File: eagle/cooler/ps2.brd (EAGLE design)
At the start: 160 x 100 mm, 8 parts, among them J1 PIN2F061.100, J2 PIN2F061.100, J3 PIN2F061.100, J4 PIN2F061.100, J5 PIN2F061.100, J6 PIN2F061.100

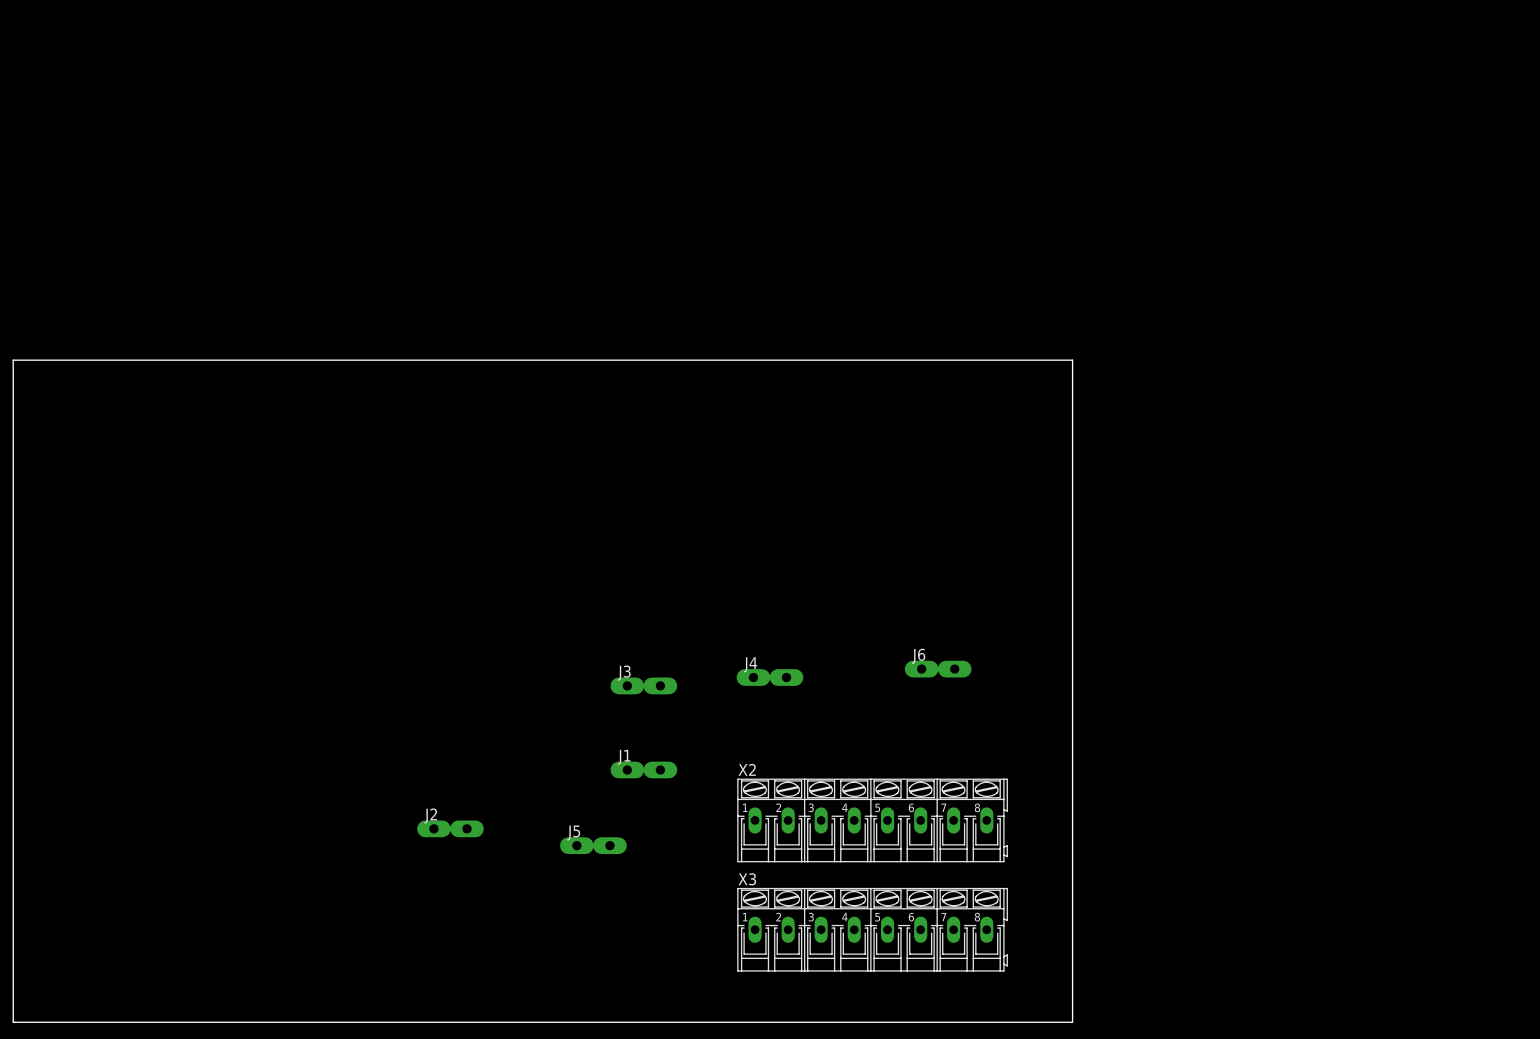
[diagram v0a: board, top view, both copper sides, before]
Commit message: layouts
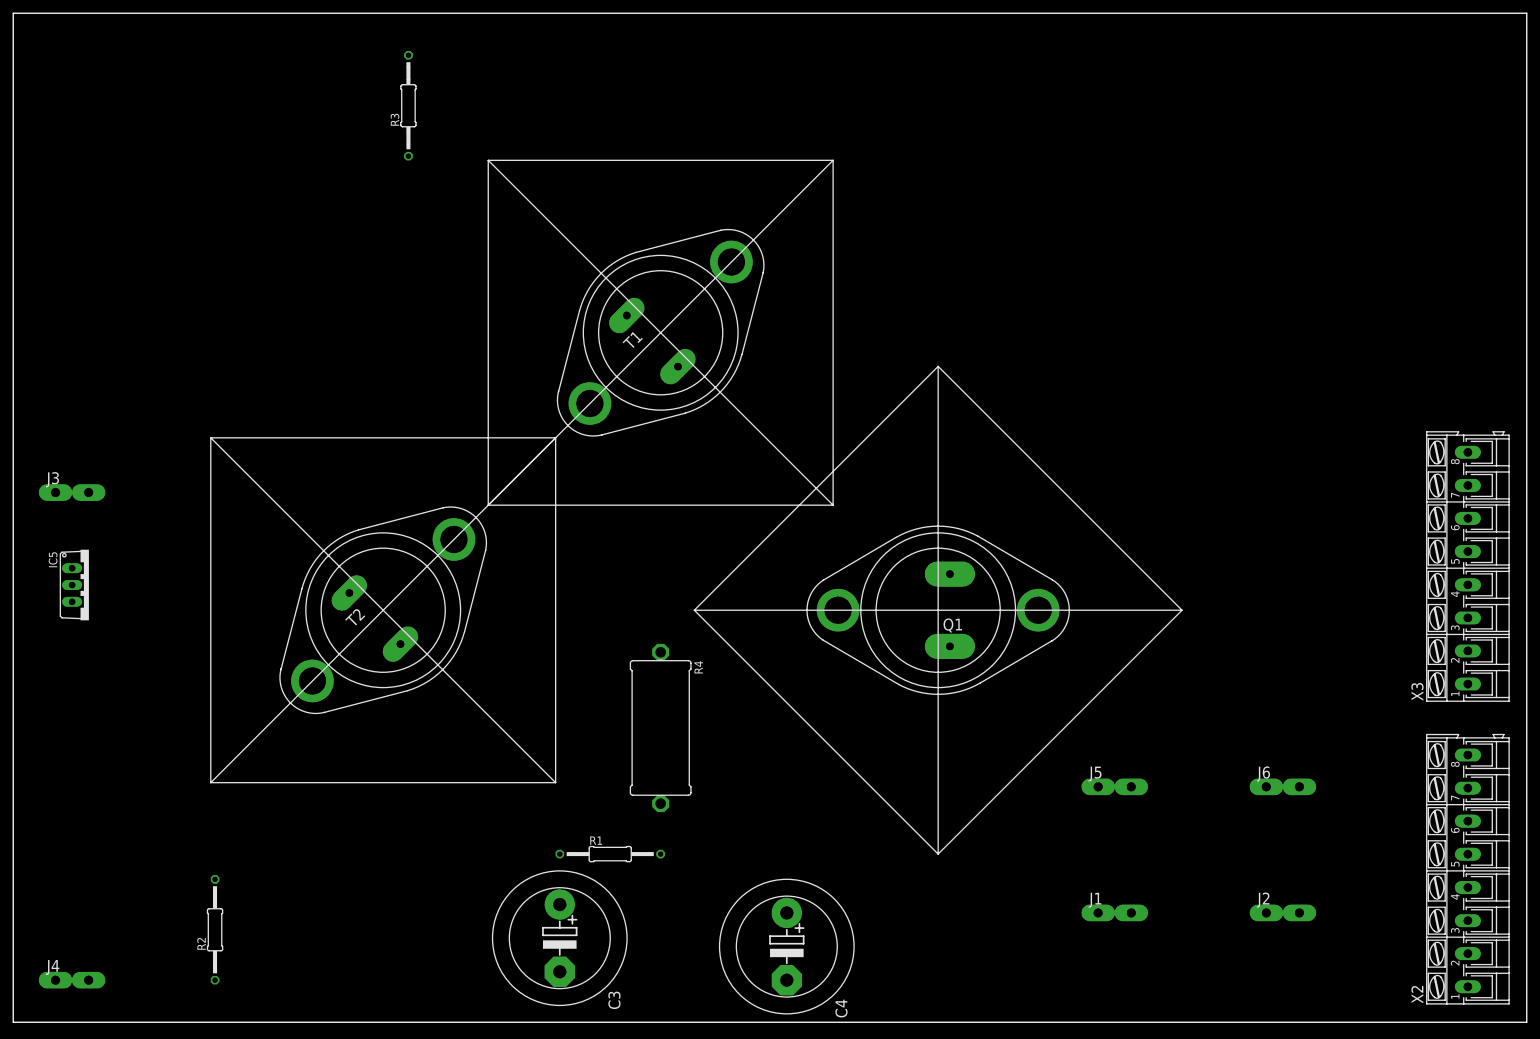
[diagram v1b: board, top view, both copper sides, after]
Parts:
- added C3, C4: 1u, rcl:EB20D
- added IC5: 7812TV, linear:TO220V
- added Q1: 2N5883, transistor-pnp:TO3
- added R1: 1K, rcl:0207/15
- added R2: 1.8K, rcl:0207/15
- added R3: 10, rcl:0207/15
- added R4: 1, rcl:0922/22
- added T1, T2: 2N3055, transistor:TO3
- moved J2 126.4 mm to (191.8, 16.5)
- moved J4 114.9 mm to (8.89, 6.35)
- moved X3 105.4 mm to (219.7, 68.6), turned to 90 degrees
- moved J3 91.2 mm to (8.89, 80.0)
- moved X2 90.5 mm to (219.7, 22.9), turned to 90 degrees
- moved J5 79.2 mm to (166.4, 35.6)
- moved J1 74.3 mm to (166.4, 16.5)
- moved J6 55.0 mm to (191.8, 35.6)
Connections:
- new net N$1: Q1.C, Q1.C/, R4.1, T1.B, T2.B
- new net N$4: IC5.1, Q1.B, R3.2
- new net N$5: IC5.2, R1.1, R2.2
- new net VIN: C3.+, J3.A1, J3.A2, Q1.E, R3.1, T1.C, T1.C/, T2.C, T2.C/
- net GND: now also C3.-, C4.-, R2.1
- net TEC1: now also X2.1, X2.3
- net TEC2: now also X2.5
- net VDD: now also C4.+, IC5.3, R1.2, R4.2, T1.E, T2.E; no longer J3.A1, J3.A2
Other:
- board size 160 x 100 mm -> 228.6 x 152.4 mm
